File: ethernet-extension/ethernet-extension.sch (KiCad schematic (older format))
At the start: 43 parts, among them J1 Wuerth_7499010121A, J2 West, J3 East, U1 W5500, Y1 25MHz

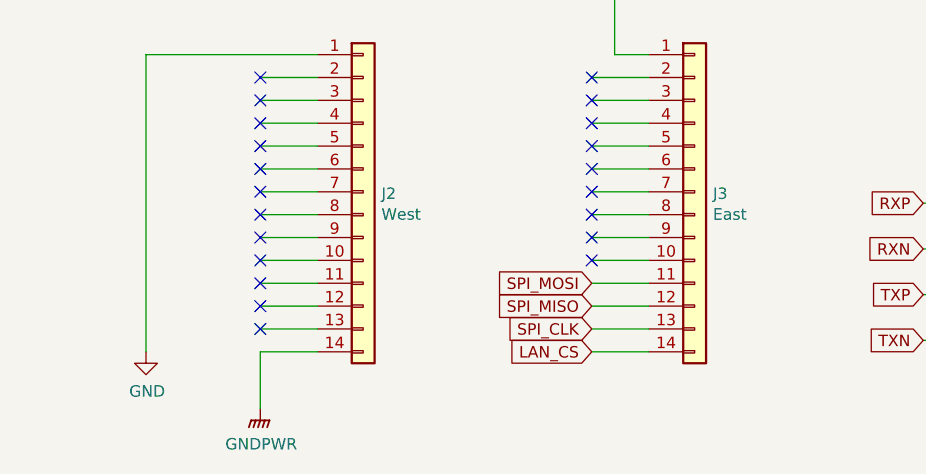
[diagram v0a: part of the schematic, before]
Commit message: Ongoing
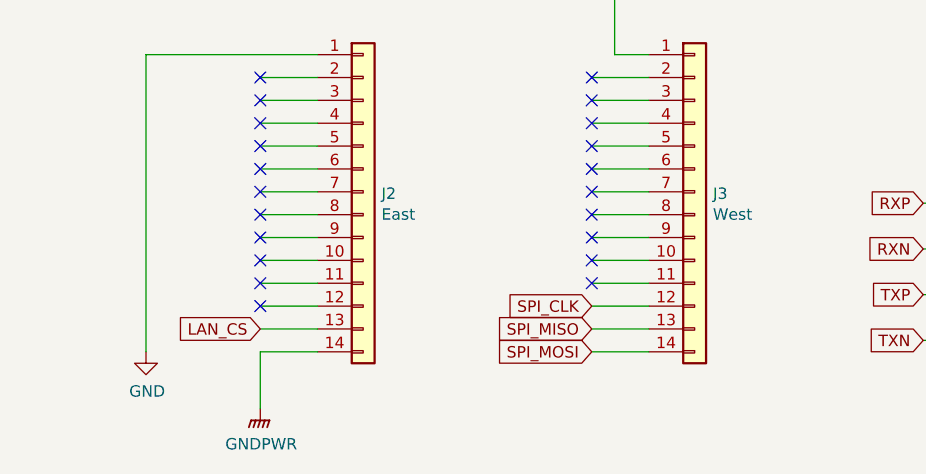
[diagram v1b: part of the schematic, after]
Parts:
- J2: value West -> East
- J3: value East -> West
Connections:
- net LAN_CS: now also J2.13 (Pin_13); no longer J3.14 (Pin_14)
- net SPI_CLK: now also J3.12 (Pin_12); no longer J3.13 (Pin_13)
- net SPI_MISO: now also J3.13 (Pin_13); no longer J3.12 (Pin_12)
- net SPI_MOSI: now also J3.14 (Pin_14); no longer J3.11 (Pin_11)
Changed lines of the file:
@@
 P 4050 6550
 F 0 "J3" H 4130 6542 50  0000 L CNN
-F 1 "East" H 4130 6451 50  0000 L CNN
+F 1 "West" H 4130 6451 50  0000 L CNN
 F 2 "Connector_PinHeader_2.54mm:PinHeader_1x14_P2.54mm_Vertical" H 4050 6550 50  0001 C CNN
 F 3 "~" H 4050 6550 50  0001 C CNN
@@
 P 2600 6550
 F 0 "J2" H 2680 6542 50  0000 L CNN
-F 1 "West" H 2680 6451 50  0000 L CNN
+F 1 "East" H 2680 6451 50  0000 L CNN
 F 2 "Connector_PinHeader_2.54mm:PinHeader_1x14_P2.54mm_Vertical" H 2600 6550 50  0001 C CNN
 F 3 "~" H 2600 6550 50  0001 C CNN
@@
 Wire Wire Line
 	1650 5950 2400 5950
+Text GLabel 2150 7150 0    50   Input ~ 0
+LAN_CS
+Text GLabel 3600 7050 0    50   Input ~ 0
+SPI_CLK
+Text GLabel 3600 7150 0    50   Input ~ 0
+SPI_MISO
 Text GLabel 3600 7250 0    50   Input ~ 0
-LAN_CS
-Text GLabel 3600 7150 0    50   Input ~ 0
-SPI_CLK
-Text GLabel 3600 7050 0    50   Input ~ 0
-SPI_MISO
-Text GLabel 3600 6950 0    50   Input ~ 0
 SPI_MOSI
 NoConn ~ 3600 6850
@@
 NoConn ~ 3600 6150
 NoConn ~ 3600 6050
-NoConn ~ 2150 7150
+NoConn ~ 3600 6950
 NoConn ~ 2150 7050
 NoConn ~ 2150 6950

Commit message: Ongoing Work
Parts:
- C11: footprint Capacitor_SMD:C_1206_3216Metric_Pad1.33x1.80mm_HandSolder -> Capacitor_SMD:C_0603_1608Metric_Pad1.08x0.95mm_HandSolder
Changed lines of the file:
@@
 F 0 "C11" V 7142 2096 50  0000 L CNN
 F 1 "10uF" V 7150 1800 50  0000 L CNN
-F 2 "Capacitor_SMD:C_1206_3216Metric_Pad1.33x1.80mm_HandSolder" H 7050 2050 50  0001 C CNN
+F 2 "Capacitor_SMD:C_0603_1608Metric_Pad1.08x0.95mm_HandSolder" H 7050 2050 50  0001 C CNN
 F 3 "~" H 7050 2050 50  0001 C CNN
 	1    7050 2050
